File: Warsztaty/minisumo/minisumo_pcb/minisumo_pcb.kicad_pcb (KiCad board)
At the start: 2 copper layers, 76.7 x 88 mm, 61 parts, among them J1 HTSW-102-08-L-S, J2 MTSW-103-23-F-S-235, M1 HTSW-102-08-L-S, M2 HTSW-102-08-L-S, Q1 PMOS, U7 LM1117S-5.0, Y1 ECS-160-20-4DN

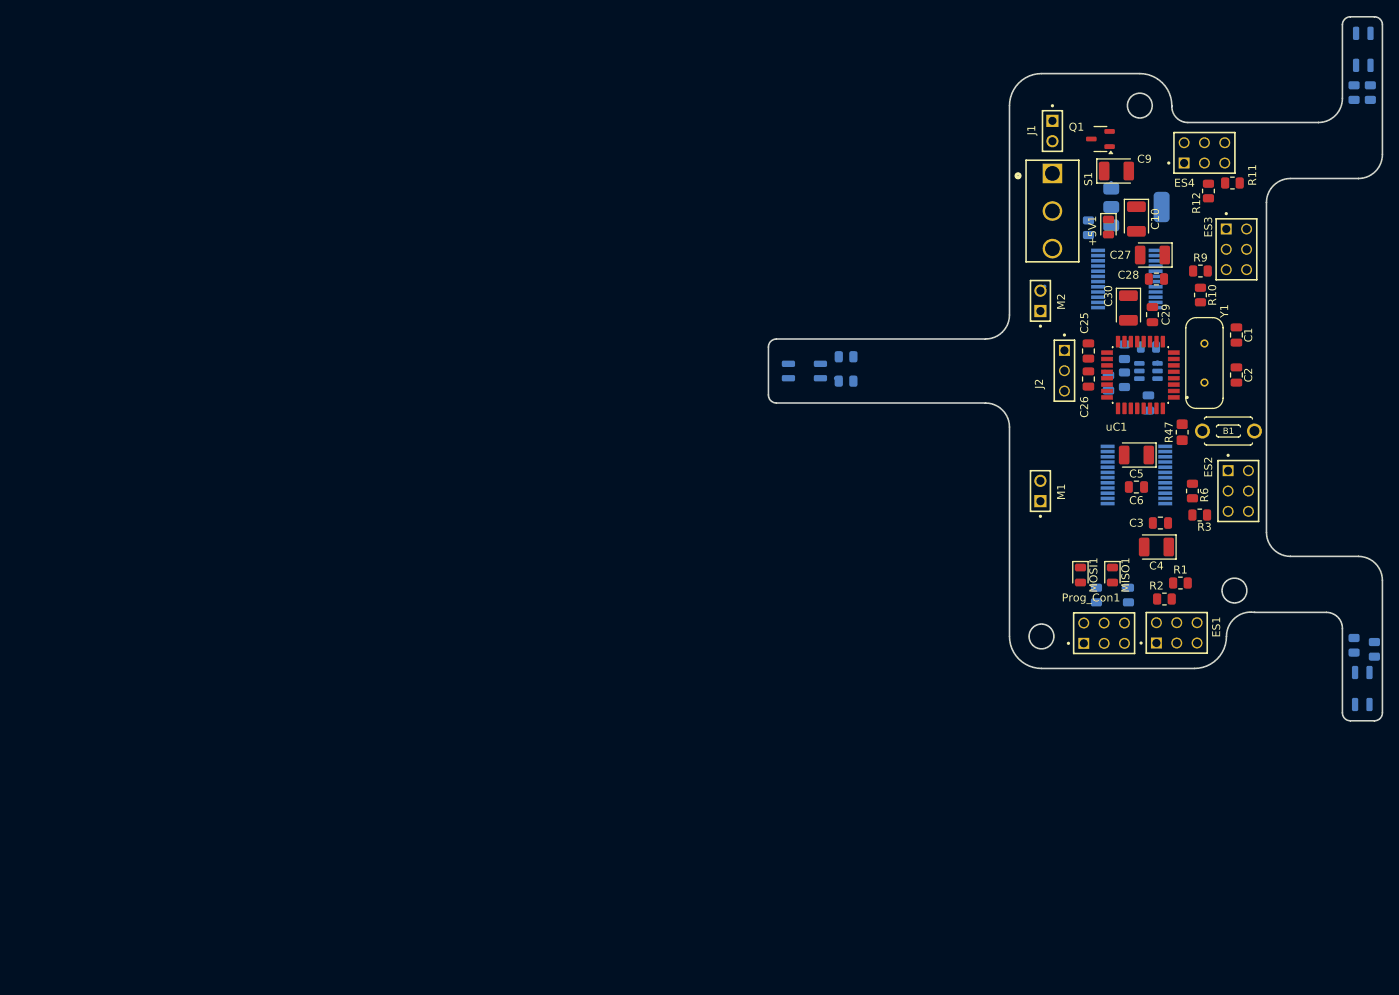
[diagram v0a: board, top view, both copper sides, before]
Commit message: koncowy projekt plytki i chyba model tez
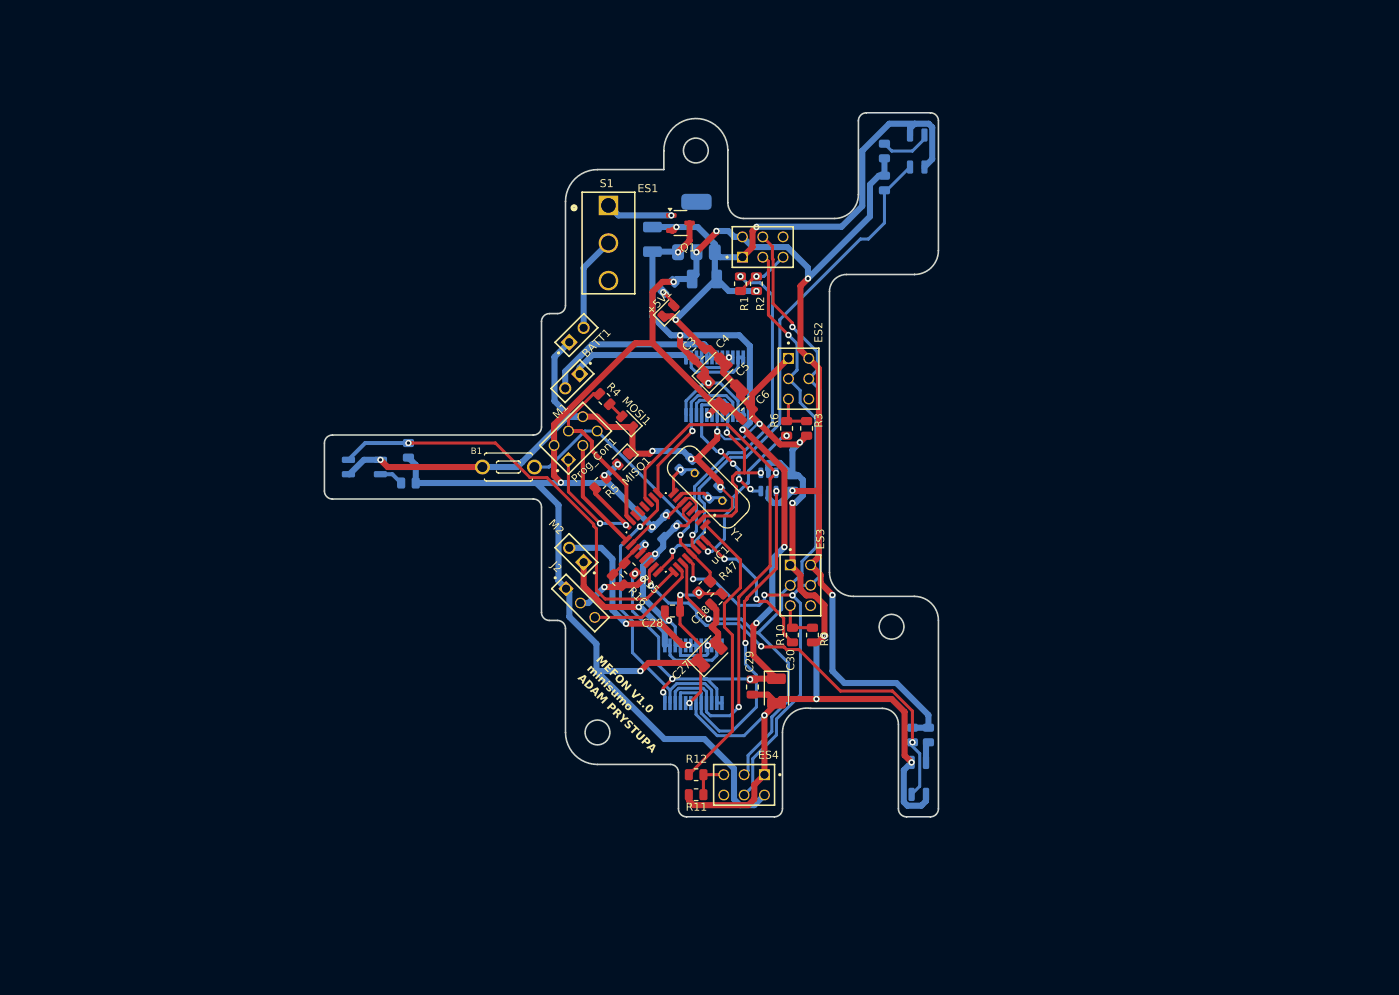
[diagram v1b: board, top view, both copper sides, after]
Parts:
- removed J1: HTSW-102-08-L-S, HTSW-102-08-L-S:SAMTEC_HTSW-102-08-L-S
- added BATT1: HTSW-102-08-L-S, HTSW-102-08-L-S:SAMTEC_HTSW-102-08-L-S, F.Cu at (138.0, 74.5)
- C1, C10, C2, C25, C26, C9: moved to B.Cu
- C18, R15, R16, R4, R5: moved to F.Cu
- moved LS1 127.8 mm to (111.5, 91.0), turned to 90 degrees
- moved R20 123.3 mm to (117.0, 88.9), turned to -90 degrees
- moved R17 119.9 mm to (117.0, 93.0), turned to 180 degrees
- moved R11 101.7 mm to (153.0, 132.0), turned to 0 degrees
- moved R12 97.1 mm to (153.0, 129.5), turned to 180 degrees
- moved ES4 92.7 mm to (161.5, 129.5), turned to 180 degrees
- moved B1 90.1 mm to (129.5, 91.0), turned to 0 degrees
- moved C27 74.5 mm to (154.6, 114.4), turned to 45 degrees
- moved C28 73.4 mm to (150.0, 109.0)
- moved M_DRIVER2 73.3 mm to (152.6, 116.9), turned to -90 degrees
- moved ES1 70.7 mm to (158.7, 64.8)
- moved C1 70.7 mm to (151.7, 90.7), turned to 45 degrees
- moved ES3 68.8 mm to (164.7, 103.2)
- moved Prog_Con1 68.4 mm to (137.0, 90.1), turned to 45 degrees
- moved C29 68.3 mm to (160.0, 118.5)
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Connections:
- Q1 pad 1: + -> +OUT
- S1 pad 1: + -> +OUT
- S1 pad 2: + -> +IN
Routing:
- net GND: track 0.00 -> 375.1 mm, vias 0 -> 23
- net +5V: track 0.39 -> 313.4 mm, vias 0 -> 14
- net +BATT: track 1.18 -> 131.8 mm, vias 0 -> 10
- net /sensor1/SCL: track 0.00 -> 96.6 mm, vias 0 -> 4
- net /sensor1/SDA: track 0.00 -> 90.6 mm, vias 0 -> 2
- net /inverter/DIRB_2: track 0.00 -> 69.6 mm, vias 0 -> 2
- net /line_sensors/LS2: track 0.00 -> 67.0 mm, vias 0 -> 1
- net /line_sensors/LS1: track 0.00 -> 56.1 mm, vias 0 -> 1
- net /line_sensors/LS3: track 0.51 -> 53.7 mm, vias 0 -> 3
- net /inverter/DIRA_2: track 0.14 -> 44.8 mm, vias 0 -> 2
- net /sensor1/X1: track 0.00 -> 42.3 mm, vias 0 -> 2
- net /motor_driver2/PWM2: track 0.00 -> 37.9 mm, vias 0 -> 1
- net /sensor4/X4: track 0.00 -> 36.6 mm
- net /programming_connector/RST: track 0.00 -> 35.2 mm, vias 0 -> 1
- net /inverter/DIRB_1: track 0.00 -> 28.4 mm, vias 0 -> 2
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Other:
- outline, holes or cut-outs redrawn
- board text added: "MEFON V1.0 minisumo ADAM PRYSTUPA"

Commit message: prawdopodobnie koncowa wersja płytki
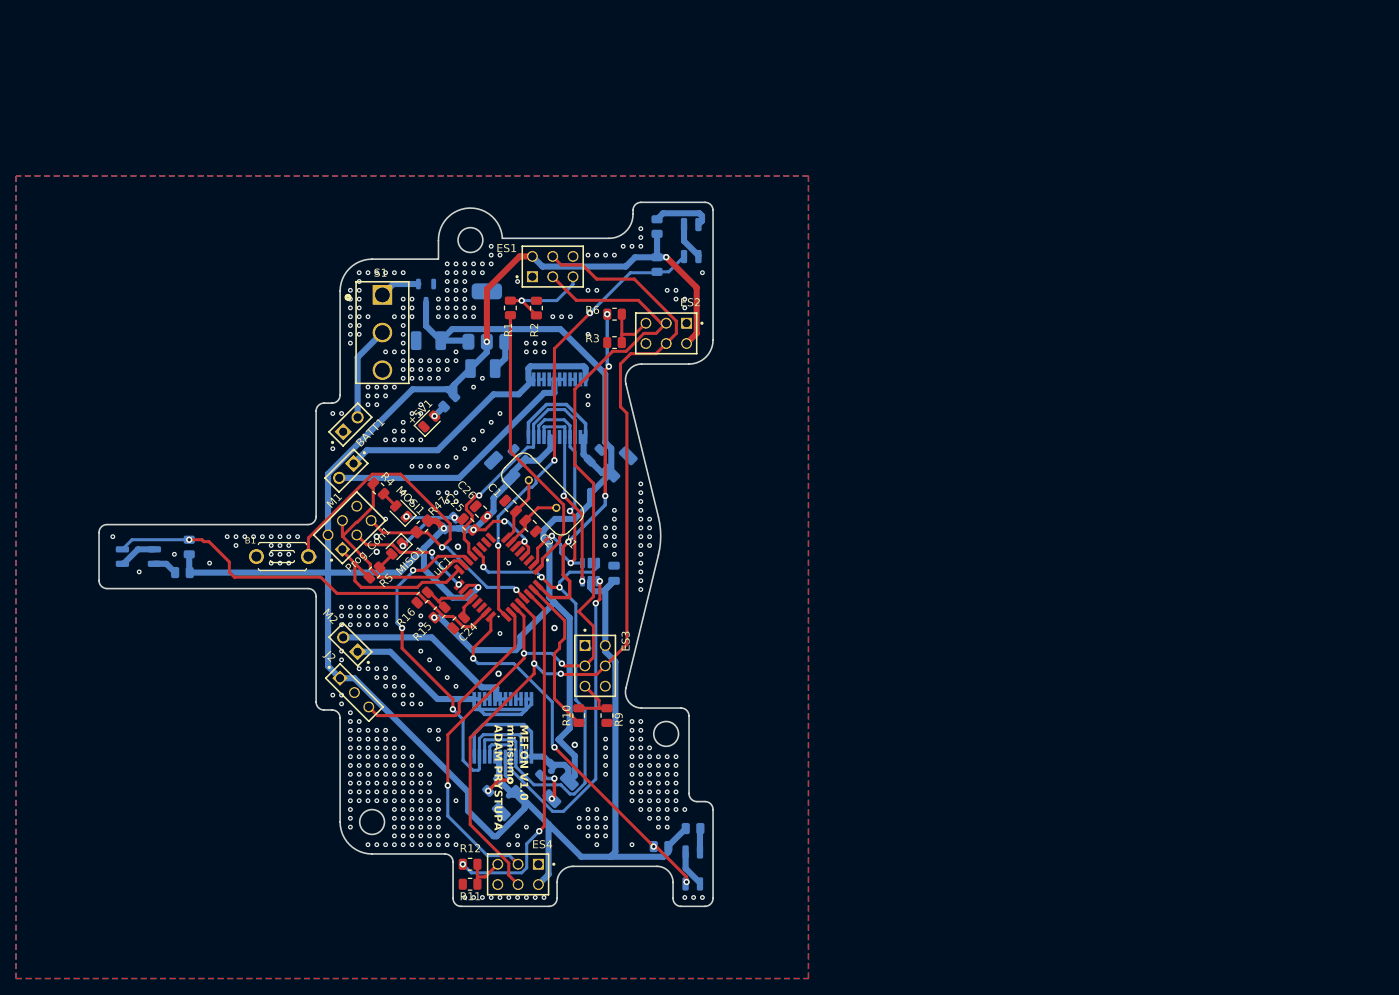
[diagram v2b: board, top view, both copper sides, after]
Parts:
- C1, C2, C24, C25, C26: moved to F.Cu
- C18, C27, C28, C29, C3, C30, C4, C5, C6, Q1: moved to B.Cu
- moved R47 36.1 mm to (118.7, 98.4), turned to 45 degrees
- moved C18 34.7 mm to (122.1, 98.0), turned to 45 degrees
- moved R14 34.4 mm to (148.6, 138.4), turned to 0 degrees
- moved Q1 33.0 mm to (119.2, 69.3), turned to -90 degrees
- moved +5V1 32.9 mm to (119.6, 85.3)
- moved R13 31.7 mm to (152.6, 136.2), turned to 0 degrees
- moved C28 31.2 mm to (127.6, 130.8), turned to -135 degrees
- moved C27 31.1 mm to (129.7, 133.0), turned to -135 degrees
- moved R7 30.9 mm to (122.1, 82.8)
- moved C9 30.7 mm to (119.5, 75.2), turned to 180 degrees
- moved R11 30.4 mm to (124.7, 143.2)
- moved R12 30.4 mm to (124.7, 140.7)
- moved B1 30.4 mm to (101.2, 102.2)
- moved BATT1 30.4 mm to (109.7, 85.7)
- moved J2 30.4 mm to (110.2, 119.2)
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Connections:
- R1 pad 2: /sensor1/X1 -> /sensor1/XSHUT_1
- R10 pad 2: /sensor3/X3 -> /sensor3/XSHUT_3
- R12 pad 2: /sensor4/X4 -> /sensor4/XSHUT_4
- R6 pad 2: /sensor2/X2 -> /sensor2/XSHUT_2
- uC1 pad 1: /sensor4/X4 -> /sensor1/XSHUT_1
- uC1 pad 10: /motor_driver2/PWM2 -> unconnected-(uC1-PD6-Pad10)
- uC1 pad 11: /inverter/DIRB_2 -> unconnected-(uC1-PD7-Pad11)
- uC1 pad 12: unconnected-(uC1-PB0-Pad12) -> /inverter/DIRB_2
- uC1 pad 13: unconnected-(uC1-PB1-Pad13) -> /motor_driver1/PWM1
- uC1 pad 14: unconnected-(uC1-PB2-Pad14) -> /motor_driver2/PWM2
- uC1 pad 23: /line_sensors/LS3 -> /line_sensors/LS1
- uC1 pad 24: /line_sensors/LS2 -> /line_sensors/LS3
- uC1 pad 25: /line_sensors/LS1 -> /line_sensors/LS2
- uC1 pad 30: /sensor1/X1 -> /sensor4/XSHUT_4
- uC1 pad 31: /sensor2/X2 -> /sensor3/XSHUT_3
- uC1 pad 32: /sensor3/X3 -> /sensor2/XSHUT_2
- uC1 pad 9: /motor_driver1/PWM1 -> unconnected-(uC1-PD5-Pad9)
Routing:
- net GND: track 375.1 -> 47.2 mm, vias 23 -> 486
- net /sensor4/XSHUT_4: track 0.00 -> 44.6 mm, vias 0 -> 2
- net /sensor2/XSHUT_2: track 0.00 -> 42.8 mm, vias 0 -> 4
- net /sensor1/X1: track 42.3 -> 0.00 mm, vias 2 -> 0
- net /sensor4/X4: track 36.6 -> 0.00 mm
- net /sensor1/XSHUT_1: track 0.00 -> 35.9 mm
- net /sensor1/SDA: track 90.6 -> 119.7 mm, vias 2 -> 3
- net /sensor1/SCL: track 96.6 -> 119.7 mm, vias 4 -> 2
- net +BATT: track 131.8 -> 153.2 mm, vias 10 -> 1
- net /sensor2/X2: track 20.4 -> 0.00 mm, vias 2 -> 0
- net /sensor3/XSHUT_3: track 0.00 -> 20.1 mm
- net /sensor3/X3: track 18.8 -> 0.00 mm, vias 2 -> 0
- net /programming_connector/RST: track 35.2 -> 53.9 mm, vias 1 -> 2
- net STARTER: track 14.4 -> 27.5 mm
- net /motor_driver2/PWM2: track 37.9 -> 50.3 mm, vias 1 -> 3
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- added copper zone on B.Cu, net GND
- added copper zone on F.Cu, net GND
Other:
- outline, holes or cut-outs redrawn
